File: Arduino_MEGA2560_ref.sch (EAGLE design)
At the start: 74 parts, among them IC1 7805DT, IC2 7805DT, T1 PHT8N06LTSOT223, T2 PHT8N06LTSOT223, T3 PHT8N06LTSOT223, T4 PHT8N06LTSOT223, T5 PHT8N06LTSOT223, T6 PHT8N06LTSOT223, X1 MKDSN1,5/2-5,08, X2 MKDSN1,5/2-5,08, X3 MKDSN1,5/2-5,08, X4 MKDSN1,5/2-5,08, X5 MKDSN1,5/2-5,08, X6 MKDSN1,5/2-5,08, X7 5566-4, X9 MKDSN1,5/2-5,08

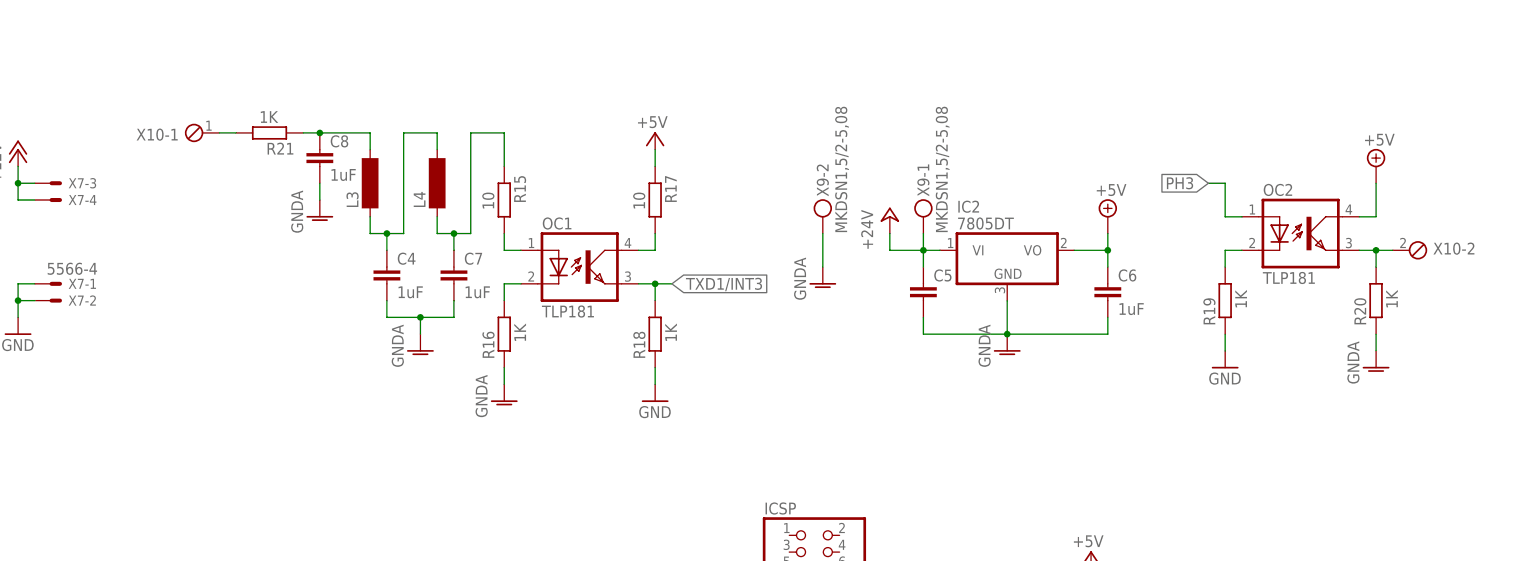
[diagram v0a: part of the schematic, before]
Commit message: done handmade
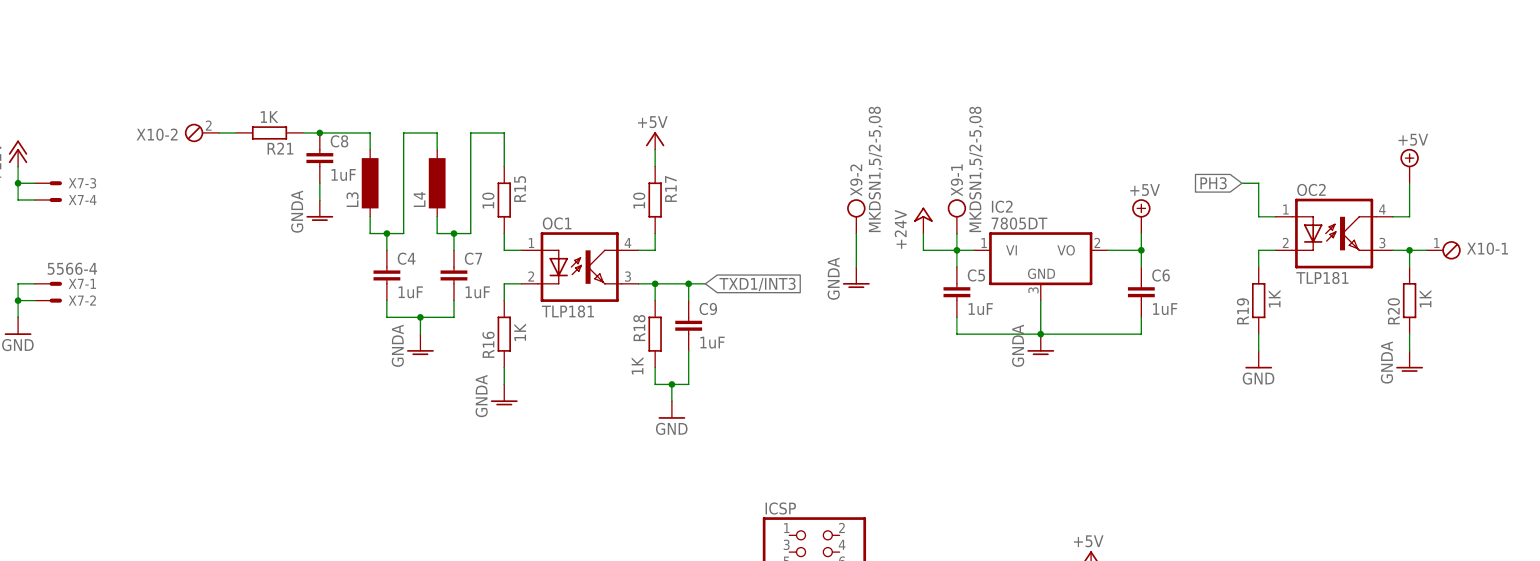
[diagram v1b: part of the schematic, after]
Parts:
- added C9: 1uF, resistor:C-EUC0805
- C5: value (none) -> 1uF
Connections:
- removed net N$19: R21.2, X10-1.1
- new net N$22: R21.2, X10-2.1
- net GND: now also C9.2
- net N$18: now also X10-1.1; no longer X10-2.1
- net TXD1/INT3: now also C9.1
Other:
- moved on the sheet: C5, C6, IC2, OC2, R19, R20, X10-1, X10-2, X9-1, X9-2

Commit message: doing factory
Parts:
- removed C7, C8: 1uF, resistor:C-EUC0805
- removed T1, T2, T3, T4, T5, T6: PHT8N06LTSOT223, NFET_transistors:PHT8N06LTSOT223
- removed X10, X11, X12, X13, X14: (no value), con-phoenix-254:MPT2
- added Q1, Q11, Q13, Q3, Q5, Q7, Q9: IRLML2502, NFET_transistors:IRLML2502
- added Q10, Q12, Q14, Q2, Q4, Q6, Q8: PF610BL, NFET_transistors:PF610BL
- added R22: 0, resistor:R-EU_M0805
- added X15, X16: 1751251, con-phoenix-350:1751251
- added X17: 1751264, con-phoenix-350:1751264
- R15: value 10 -> 1K
- R16: value 1K -> 0
- X8: value (none) -> 1751248; device con-phoenix-254:MPT2 -> con-phoenix-350:1751248
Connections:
- net +5V: now also R15.1, X15-2.K, X16-2.K; no longer X11-1.1, X13-2.1
- net GND: now also Q1.S, Q10.S, Q11.S, Q12.S, Q2.S, Q3.S, Q4.S, Q5.S, Q6.S, Q7.S, Q8.S, Q9.S, R16.2, R22.2, X15-1.K, X16-3.K, X17-1.K, X17-2.K; no longer T1.S, T2.S, T3.S, T4.S, T5.S, T6.S, X11-2.1, X13-1.1, X14-1.1, X8-1.1
- net GNDA: now also Q13.S, Q14.S, R22.1; no longer C7.2, C8.2
- net N$1: now also Q11.G, Q12.G; no longer T1.G
- net N$10: now also Q1.D, Q2.D; no longer T5.D
- net N$11: now also Q5.G, Q6.G; no longer T6.G
- net N$12: now also Q5.D, Q6.D; no longer T6.D
- net N$14: now also Q13.D, Q14.D; no longer R16.2
- net N$17: no longer C8.1
- net N$18: now also X8-1.K; no longer X10-1.1
- net N$2: now also Q10.G, Q9.G; no longer T2.G
- net N$21: now also Q13.G, Q14.G; no longer C7.1, R15.1
- net N$22: now also X8-2.K; no longer X10-2.1
- net N$3: now also Q3.G, Q4.G; no longer T4.G
- net N$4: now also Q11.D, Q12.D; no longer T1.D
- net N$5: now also Q7.G, Q8.G; no longer T3.G
- net N$6: now also Q10.D, Q9.D; no longer T2.D
- net N$7: now also Q7.D, Q8.D; no longer T3.D
- net N$8: now also Q3.D, Q4.D; no longer T4.D
- net N$9: now also Q1.G, Q2.G; no longer T5.G
- net PB4: now also X15-3.K; no longer X12-2.1
- net PB6: now also X17-3.K; no longer X14-2.1
- net PB7: now also X17-4.K; no longer X8-2.1
- net PH6: now also X16-1.K; no longer X12-1.1
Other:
- moved on the sheet: C1, C2, C4, D1, D2, D3, D4, D5, D6, L3, L4, PWMH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
